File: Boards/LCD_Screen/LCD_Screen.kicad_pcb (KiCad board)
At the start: 2 copper layers, 65 x 34 mm, 32 parts, among them J1 MicroFit_VT_4, U1 MCP25625-x-SS, U2 Raspberry_Pi_Zero, U3 TPS563231, Y1 Crystal_SMD

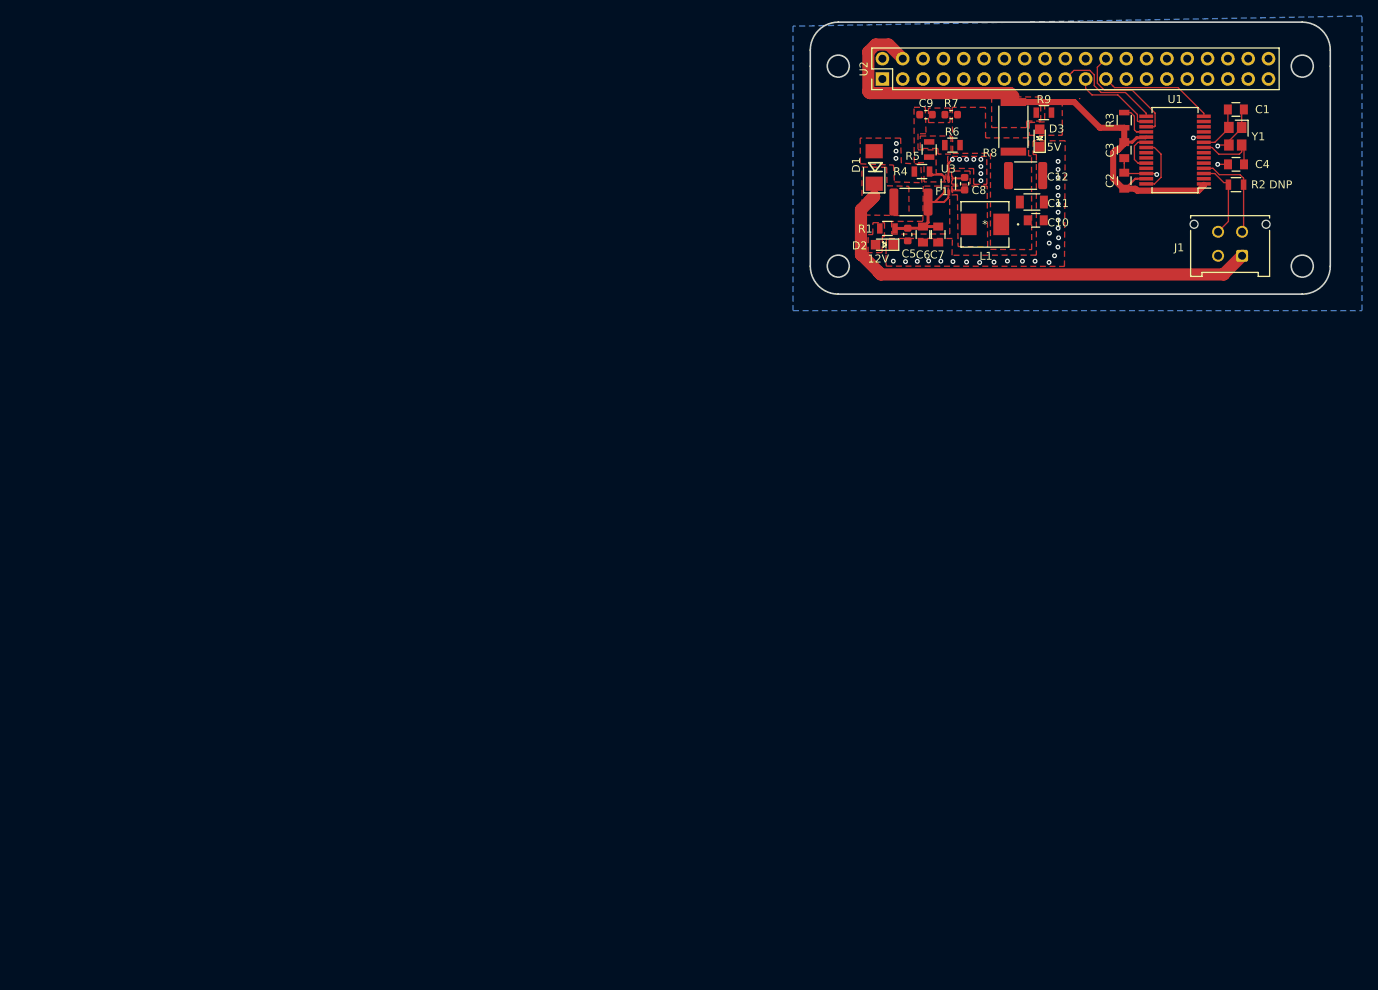
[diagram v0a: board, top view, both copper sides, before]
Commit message: Revert "Begin Layout"
This reverts commit f66e97611986f6cb10e89dffa2fa205961dd2a3d.
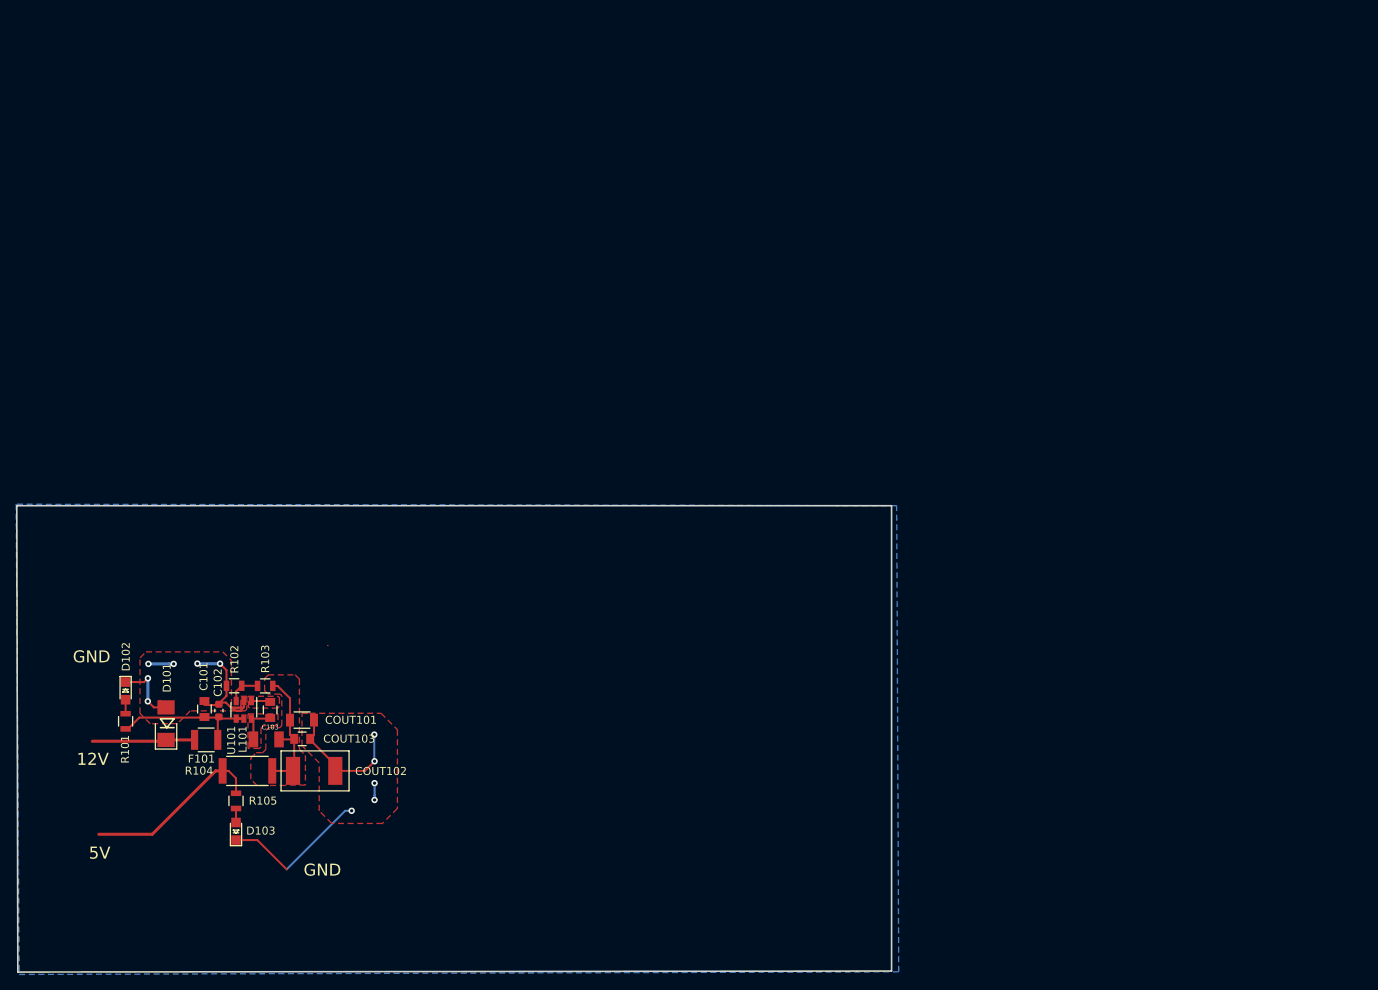
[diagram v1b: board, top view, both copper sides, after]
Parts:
- removed C1, C4: C_30pF, footprints:C_0805_OEM
- removed C10: C_10uF, footprints:C_0805_OEM
- removed C11: C_22uF, footprints:C_1206_OEM
- removed C12: C_33uF, footprints:C_1812_4532Metric
- removed C2: C_0.1uF, footprints:C_0805_OEM
- removed C3: C_100pF, footprints:C_0805_OEM
- removed C5: C_0.1uF, footprints:C_0603_1608Metric
- removed C6, C7: C_10uF_25V, footprints:C_0805_OEM
- removed C8: C_0.1uF_0603, footprints:C_0603_1608Metric
- removed C9: C_100nF, footprints:C_0603_1608Metric
- removed D1: D_Zener_18V, footprints:DO-214AA
- removed D2, D3: LED_0805, footprints:LED_0805_OEM
- removed F1: F_2.6A_16V, footprints:Fuse_1812_4532Metric
- removed J1: MicroFit_VT_4, footprints:MicroFit_VT_4
- removed L1: L_4.7uH_3.2A, footprints:IHLP2020BZER4R7M11
- removed R1: R_1K, footprints:R_0805_OEM
- removed R2: R_120_DNP, footprints:R_0805_OEM
- removed R3, R4: R_10K, footprints:R_0805_OEM
- removed R5: R_51.1K, footprints:R_0805_OEM
- removed R6: R_22K, footprints:R_0805_OEM
- removed R7: R_1, footprints:R_0603_1608Metric
- removed R8: R_0_2512, footprints:R_2512_OEM
- removed R9: R_200, footprints:R_0805_OEM
- removed U1: MCP25625-x-SS, Package_SO:SSOP-28_5.3x10.2mm_P0.65mm
- removed U2: Raspberry_Pi_Zero, footprints:PinHeader_2x20_P2.54mm_Vertical
- removed U3: TPS563231, footprints:SOT-563
- removed Y1: Crystal_SMD, footprints:Crystal_SMD_FA238
- added C101: C_0.1uF, footprints:C_0805_OEM, F.Cu at (121.8, 101.9)
- added C102: C_2.2uF, footprints:C_0603_1608Metric, F.Cu at (123.6, 102.1)
- added C103: C_0.1uF, footprints:C_0805_OEM, F.Cu at (130.0, 102.0)
- added COUT101: C_22uF, footprints:C_1206_OEM, F.Cu at (133.9, 103.3)
- added COUT102: C_33uF, footprints:Fuse_1812, F.Cu at (132.8, 109.6)
- added COUT103: C_47uF, footprints:C_0805_OEM, F.Cu at (134.0, 105.6)
- added D101: D_Zener_18V, footprints:DO-214AA, F.Cu at (117.0, 103.7)
- added D102: LED_0805, footprints:LED_0805_OEM, F.Cu at (111.9, 99.6)
- added D103: LED_0805, footprints:LED_0805_OEM, F.Cu at (125.7, 117.2)
- added F101: F_500mA_16V, footprints:Fuse_1210, F.Cu at (122.0, 105.7)
- added G***: LOGO, footprints:phoenix, B.Cu at (179.6, 107.2)
- added L101: L_100uH, footprints:L_100uH, F.Cu at (129.5, 105.7)
- added R101: R_200, footprints:R_0805_OEM, F.Cu at (111.9, 103.4)
- added R102: R_25K, footprints:R_0805_OEM, F.Cu at (125.5, 99.0)
- added R103: R_100K, footprints:R_0805_OEM, F.Cu at (129.3, 99.0)
- added R104: R_0_2512, footprints:R_2512_OEM, F.Cu at (127.1, 109.6)
- added R105: R_200, footprints:R_0805_OEM, F.Cu at (125.7, 113.3)
- added U101: TPS560430YF, footprints:SOT-23-6_OEM, F.Cu at (126.7, 102.0)
- moved G*** 121.3 mm to (121.2, 85.1)
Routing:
- net VCC: track 83.4 -> 22.7 mm
- net /12V: track 68.3 -> 12.9 mm
- net GND: track 17.9 -> 65.5 mm, vias 42 -> 11
- net Net-(C101-Pad1): track 0.00 -> 18.1 mm
- net Net-(COUT101-Pad1): track 0.00 -> 17.3 mm
- net Net-(C5-Pad1): track 15.2 -> 0.00 mm
- net /~CS~: track 15.0 -> 0.00 mm
- net /SCK: track 14.4 -> 0.00 mm
- net /MOSI: track 13.9 -> 0.00 mm
- net /CANH: track 12.3 -> 0.00 mm
- net /MISO: track 11.0 -> 0.00 mm
- net /CANL: track 9.90 -> 0.00 mm
- net Net-(C4-Pad1): track 8.74 -> 0.00 mm
- net Net-(U1-Pad21): track 7.28 -> 0.00 mm
- net Net-(C1-Pad1): track 6.26 -> 0.00 mm
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- added copper zone on F.Cu, net Net-(C103-Pad1)
- added copper zone on F.Cu, net Net-(C103-Pad2)
- added copper zone on F.Cu, net Net-(COUT101-Pad1)
- removed copper zone on F.Cu, net /12V
- removed copper zone on F.Cu, net Net-(C10-Pad1)
- removed copper zone on F.Cu, net Net-(C5-Pad1)
- removed copper zone on F.Cu, net Net-(C8-Pad1)
- removed copper zone on F.Cu, net Net-(C8-Pad2)
- removed copper zone on F.Cu, net Net-(C9-Pad1)
- removed copper zone on F.Cu, net Net-(C9-Pad2)
- removed copper zone on F.Cu, net Net-(D2-Pad2)
- removed copper zone on F.Cu, net Net-(D3-Pad2)
- removed copper zone on F.Cu, net Net-(R5-Pad1)
- removed copper zone on F.Cu, net VCC
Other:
- board size 65 x 34 mm -> 109.3 x 58.3 mm
- board text added: "GND"
- board text removed: "1/11/2020"
- board text removed: "DNP"
- board text removed: "Jackie Zeng"
- board text removed: "LCD Board Rev 1"
- board text removed: "RaspPi goes on this side"

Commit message: Begin Layout
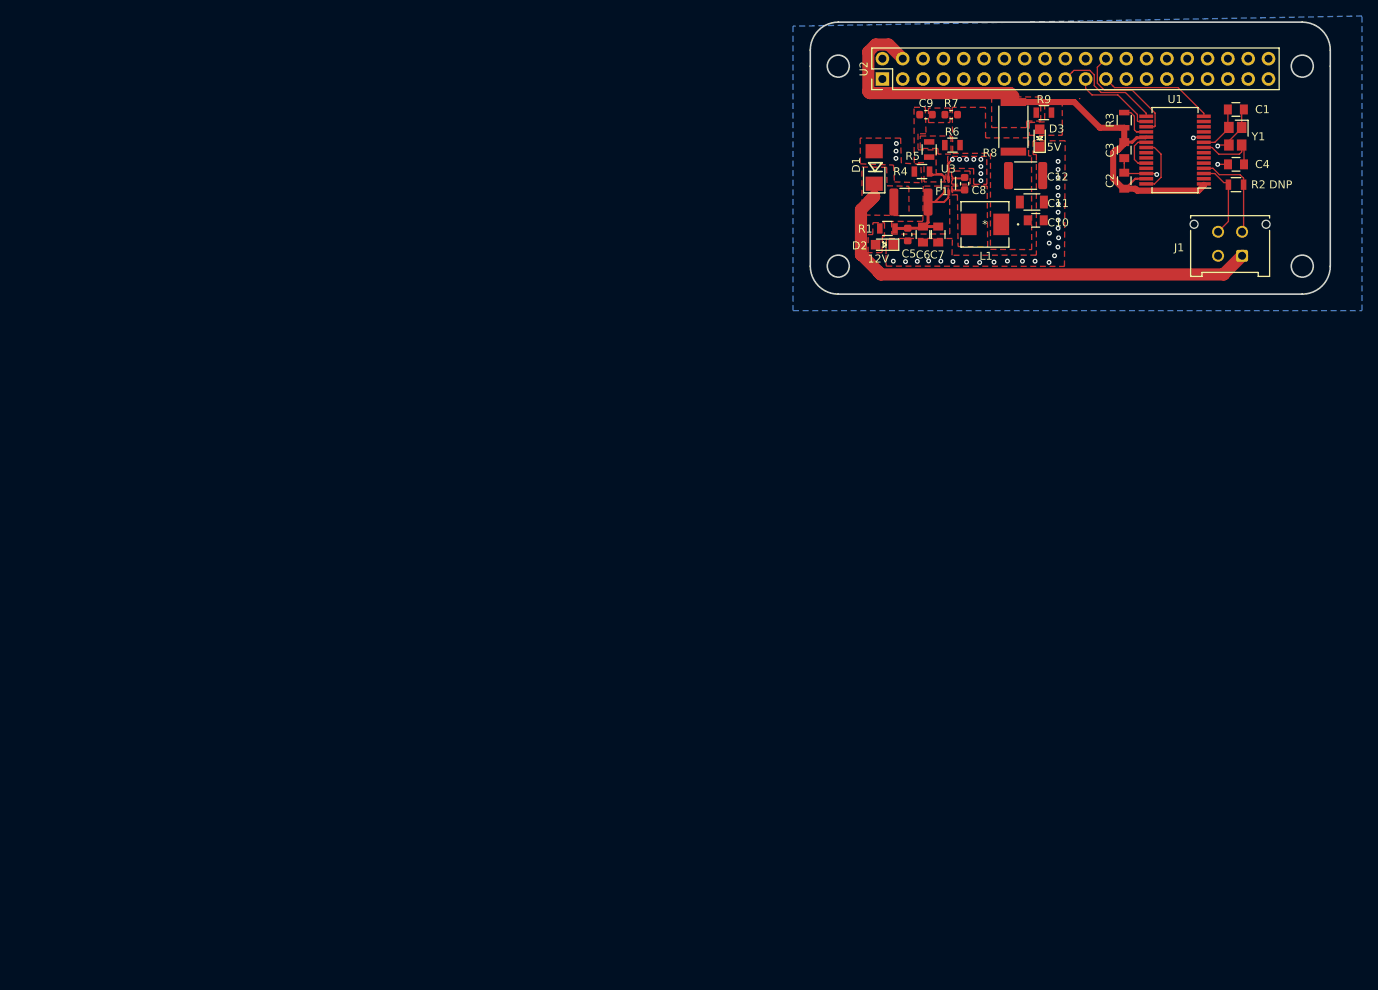
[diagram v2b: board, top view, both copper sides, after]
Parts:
- removed C101, C103: C_0.1uF, footprints:C_0805_OEM
- removed C102: C_2.2uF, footprints:C_0603_1608Metric
- removed COUT101: C_22uF, footprints:C_1206_OEM
- removed COUT102: C_33uF, footprints:Fuse_1812
- removed COUT103: C_47uF, footprints:C_0805_OEM
- removed D101: D_Zener_18V, footprints:DO-214AA
- removed D102, D103: LED_0805, footprints:LED_0805_OEM
- removed F101: F_500mA_16V, footprints:Fuse_1210
- removed the G*** at (179.6, 107.2)
- removed L101: L_100uH, footprints:L_100uH
- removed R101, R105: R_200, footprints:R_0805_OEM
- removed R102: R_25K, footprints:R_0805_OEM
- removed R103: R_100K, footprints:R_0805_OEM
- removed R104: R_0_2512, footprints:R_2512_OEM
- removed U101: TPS560430YF, footprints:SOT-23-6_OEM
- added C1: C_30pF, footprints:C_0805_OEM, F.Cu at (250.7, 26.9)
- added C10: C_10uF, footprints:C_0805_OEM, F.Cu at (225.7, 40.8)
- added C11: C_22uF, footprints:C_1206_OEM, F.Cu at (225.2, 38.5)
- added C12: C_33uF, footprints:C_1812_4532Metric, F.Cu at (224.4, 35.2)
- added C2: C_0.1uF, footprints:C_0805_OEM, F.Cu at (236.7, 35.8)
- added C3: C_100pF, footprints:C_0805_OEM, F.Cu at (236.7, 32.0)
- added C4: C_30pF, footprints:C_0805_OEM, F.Cu at (250.7, 33.8)
- added C5: C_0.1uF, footprints:C_0603_1608Metric, F.Cu at (209.7, 42.6)
- added C6: C_10uF_25V, footprints:C_0805_OEM, F.Cu at (211.6, 42.6)
- added C7: C_10uF_25V, footprints:C_0805_OEM, F.Cu at (213.5, 42.6)
- added C8: C_0.1uF_0603, footprints:C_0603_1608Metric, F.Cu at (216.8, 36.2)
- added C9: C_100nF, footprints:C_0603_1608Metric, F.Cu at (212.0, 27.6)
- added D1: D_Zener_18V, footprints:DO-214AA, F.Cu at (205.5, 34.2)
- added D2: LED_0805, footprints:LED_0805_OEM, F.Cu at (206.7, 43.8)
- added D3: LED_0805, footprints:LED_0805_OEM, F.Cu at (226.2, 30.5)
- added F1: F_2.6A_16V, footprints:Fuse_1812_4532Metric, F.Cu at (210.1, 38.5)
- added J1: MicroFit_VT_4, footprints:MicroFit_VT_4, F.Cu at (251.5, 45.2)
- added L1: L_4.7uH_3.2A, footprints:IHLP2020BZER4R7M11, F.Cu at (219.3, 41.3)
- added R1: R_1K, footprints:R_0805_OEM, F.Cu at (207.1, 41.8)
- added R2: R_120_DNP, footprints:R_0805_OEM, F.Cu at (250.7, 36.3)
- added R3: R_10K, footprints:R_0805_OEM, F.Cu at (236.7, 28.3)
- added R4: R_10K, footprints:R_0805_OEM, F.Cu at (211.4, 34.7)
- added R5: R_51.1K, footprints:R_0805_OEM, F.Cu at (212.3, 31.9)
- added R6: R_22K, footprints:R_0805_OEM, F.Cu at (215.3, 31.4)
- added R7: R_1, footprints:R_0603_1608Metric, F.Cu at (215.1, 27.6)
- added R8: R_0_2512, footprints:R_2512_OEM, F.Cu at (222.9, 29.1)
- added R9: R_200, footprints:R_0805_OEM, F.Cu at (226.7, 27.3)
- added U1: MCP25625-x-SS, Package_SO:SSOP-28_5.3x10.2mm_P0.65mm, F.Cu at (243.1, 32.0)
- added U2: Raspberry_Pi_Zero, footprints:PinHeader_2x20_P2.54mm_Vertical, F.Cu at (206.5, 23.1)
- added U3: TPS563231, footprints:SOT-563, F.Cu at (214.7, 36.3)
- added Y1: Crystal_SMD, footprints:Crystal_SMD_FA238, F.Cu at (250.6, 30.3)
- moved G*** 121.3 mm to (230.9, 33.3)
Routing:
- net VCC: track 22.7 -> 83.4 mm
- net /12V: track 12.9 -> 68.3 mm
- net GND: track 65.5 -> 17.9 mm, vias 11 -> 42
- net Net-(C101-Pad1): track 18.1 -> 0.00 mm
- net Net-(COUT101-Pad1): track 17.3 -> 0.00 mm
- net Net-(C5-Pad1): track 0.00 -> 15.2 mm
- net /~CS~: track 0.00 -> 15.0 mm
- net /SCK: track 0.00 -> 14.4 mm
- net /MOSI: track 0.00 -> 13.9 mm
- net /CANH: track 0.00 -> 12.3 mm
- net /MISO: track 0.00 -> 11.0 mm
- net /CANL: track 0.00 -> 9.90 mm
- net Net-(C4-Pad1): track 0.00 -> 8.74 mm
- net Net-(U1-Pad21): track 0.00 -> 7.28 mm
- net Net-(C1-Pad1): track 0.00 -> 6.26 mm
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- added copper zone on F.Cu, net /12V
- added copper zone on F.Cu, net Net-(C10-Pad1)
- added copper zone on F.Cu, net Net-(C5-Pad1)
- added copper zone on F.Cu, net Net-(C8-Pad1)
- added copper zone on F.Cu, net Net-(C8-Pad2)
- added copper zone on F.Cu, net Net-(C9-Pad1)
- added copper zone on F.Cu, net Net-(C9-Pad2)
- added copper zone on F.Cu, net Net-(D2-Pad2)
- added copper zone on F.Cu, net Net-(D3-Pad2)
- added copper zone on F.Cu, net Net-(R5-Pad1)
- added copper zone on F.Cu, net VCC
- removed copper zone on F.Cu, net Net-(C103-Pad1)
- removed copper zone on F.Cu, net Net-(C103-Pad2)
- removed copper zone on F.Cu, net Net-(COUT101-Pad1)
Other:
- board size 109.3 x 58.3 mm -> 65 x 34 mm
- board text added: "1/11/2020"
- board text added: "DNP"
- board text added: "Jackie Zeng"
- board text added: "LCD Board Rev 1"
- board text added: "RaspPi goes on this side"
- board text removed: "GND"
